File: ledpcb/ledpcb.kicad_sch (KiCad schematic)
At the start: 14 parts, among them J1 Conn_01x02_Female, J2 Conn_01x04_Female, J3 Barrel_Jack, J4 Conn_01x04_Male, Q1 ME2306A, Q2 ME2306A, Q3 ME2306A, SW1 SW_Push, U1 SPX3819M5-L-3-3_TR, U2 ESP32-WROOM-32, U3 TMP100

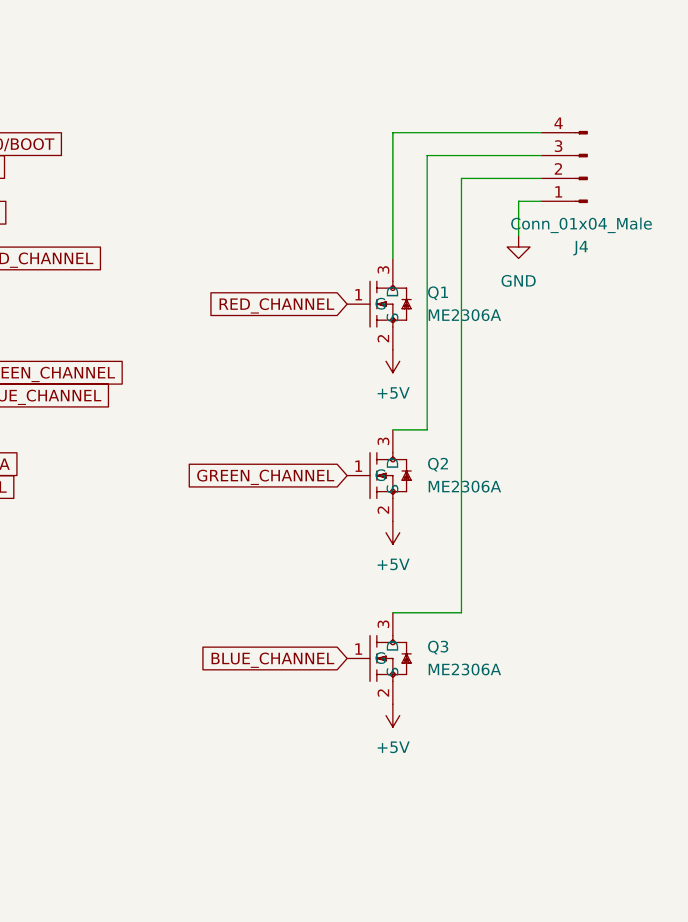
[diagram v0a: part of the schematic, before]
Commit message: progress
Signed-off-by: 3nt3 <gott@3nt3.de>
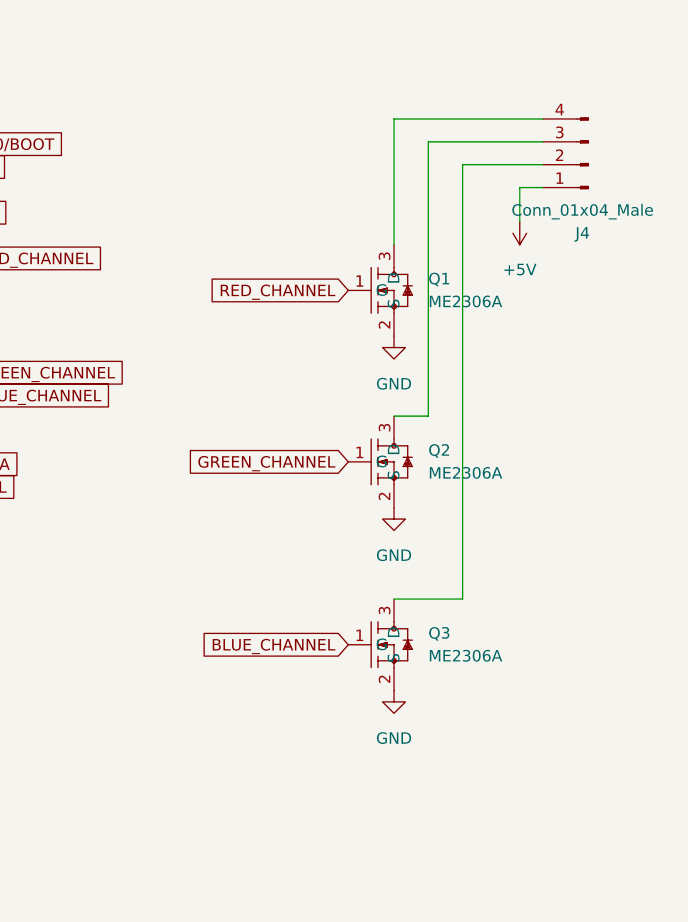
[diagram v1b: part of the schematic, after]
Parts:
- J1: footprint (none) -> Connector_PinHeader_1.27mm:PinHeader_1x02_P1.27mm_Vertical
- J2: footprint (none) -> Connector_PinHeader_2.00mm:PinHeader_1x04_P2.00mm_Horizontal
- J3: footprint (none) -> Library:DEALON DC-S050-200
- R2, R3: footprint (none) -> Resistor_SMD:R_0603_1608Metric_Pad0.98x0.95mm_HandSolder
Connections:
- net +5V: now also J4.1 (Pin_1); no longer Q1.2 (S), Q2.2 (S), Q3.2 (S)
- net GND: now also Q1.2 (S), Q2.2 (S), Q3.2 (S); no longer J4.1 (Pin_1)
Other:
- moved on the sheet: J4, Q1, Q2, Q3
